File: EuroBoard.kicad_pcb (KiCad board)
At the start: 2 copper layers, 99.9 x 99.9 mm, 36 parts, among them J1 GPIO, J10 PD1, J11 PD2, J12 PD3, J2 Conn_01x07_Male, J3 I2C, J4 Conn_01x05_Male, J5 RX, J6 TX, J7 GND, SW1 RESET, SW2 SW_DIP_x04, U1 AMS1117-3.3, U2 STM32G030CxT, Y1 NX2520 16MHz

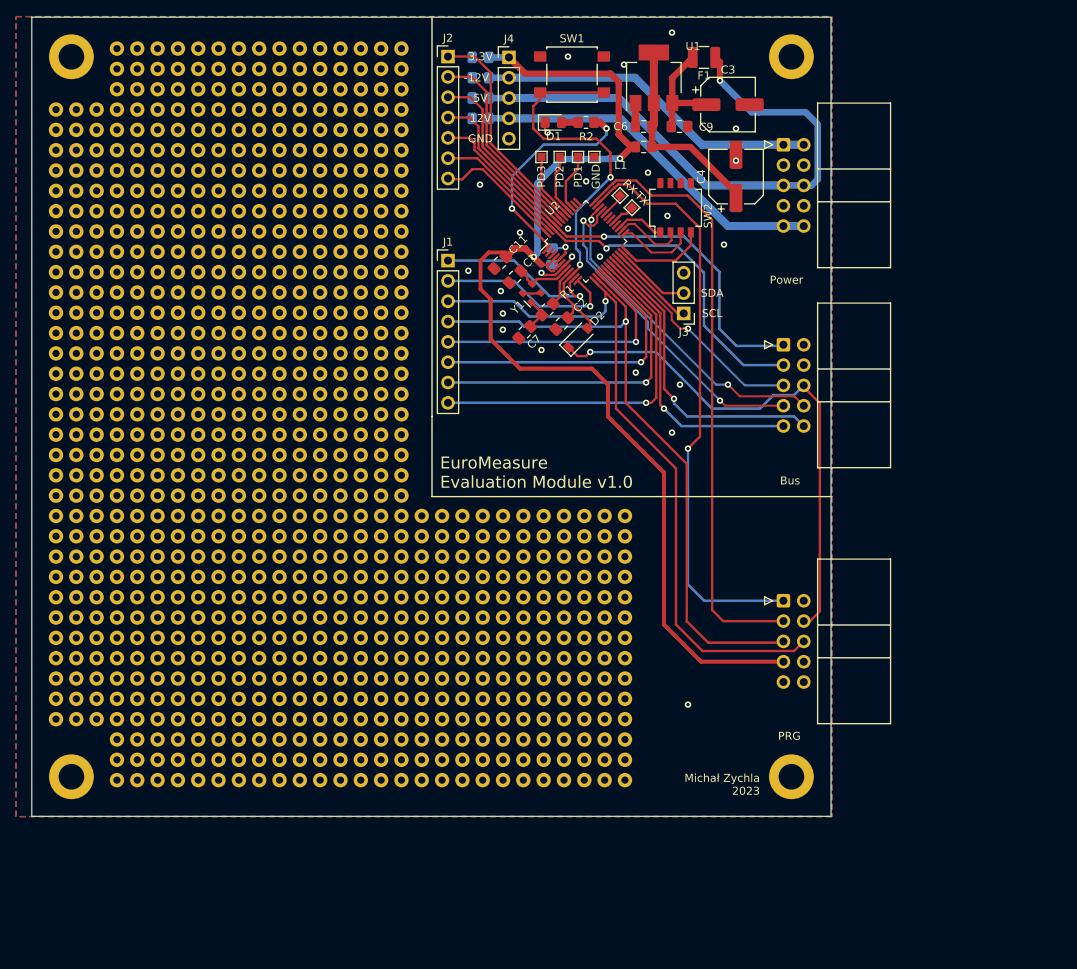
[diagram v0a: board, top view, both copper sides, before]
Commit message: Rework
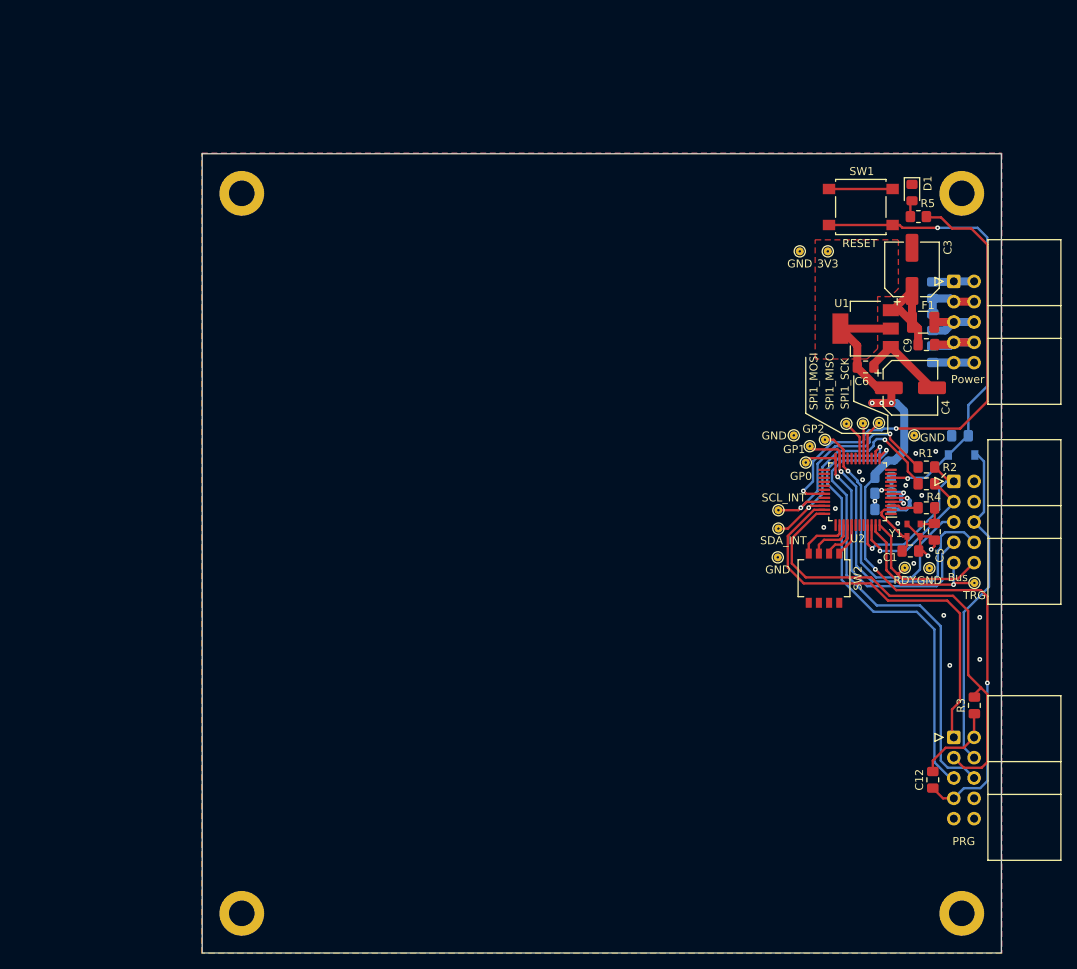
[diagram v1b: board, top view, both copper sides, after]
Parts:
- removed C11: 10u, Capacitor_SMD:C_0805_2012Metric_Pad1.18x1.45mm_HandSolder
- removed J1: GPIO, Connector_PinHeader_2.54mm:PinHeader_1x08_P2.54mm_Vertical
- removed J10: PD1, TestPoint:TestPoint_Pad_1.0x1.0mm
- removed J11: PD2, TestPoint:TestPoint_Pad_1.0x1.0mm
- removed J12: PD3, TestPoint:TestPoint_Pad_1.0x1.0mm
- removed J2: Conn_01x07_Male, Connector_PinHeader_2.54mm:PinHeader_1x07_P2.54mm_Vertical
- removed J3: I2C, Connector_PinHeader_2.54mm:PinHeader_1x03_P2.54mm_Vertical
- removed J4: Conn_01x05_Male, Connector_PinHeader_2.54mm:PinHeader_1x05_P2.54mm_Vertical
- removed J5: RX, TestPoint:TestPoint_Pad_1.0x1.0mm
- removed J6: TX, TestPoint:TestPoint_Pad_1.0x1.0mm
- removed J7: GND, TestPoint:TestPoint_Pad_1.0x1.0mm
- removed REF**: ProtoArea, MEMS_Custom:ProtoArea
- added C5: 8p, Capacitor_SMD:C_0805_2012Metric_Pad1.18x1.45mm_HandSolder, F.Cu at (187.8, 97.4)
- added R3: 10k, Capacitor_SMD:C_0805_2012Metric_Pad1.18x1.45mm_HandSolder, F.Cu at (192.8, 119.1)
- added R4: 0R, Capacitor_SMD:C_0805_2012Metric_Pad1.18x1.45mm_HandSolder, F.Cu at (186.8, 94.4)
- added R5: 1k, Resistor_SMD:R_0805_2012Metric_Pad1.20x1.40mm_HandSolder, F.Cu at (185.8, 58.0)
- added TP1: SPI1_SCK, MEMS_Custom:TestPoint_Pad_D1.0mm, F.Cu at (180.9, 83.8)
- added TP10: GP0, MEMS_Custom:TestPoint_Pad_D1.0mm, F.Cu at (171.7, 88.7)
- added TP11: GND, MEMS_Custom:TestPoint_Pad_D1.0mm, F.Cu at (168.2, 100.6)
- added TP12: GND, MEMS_Custom:TestPoint_Pad_D1.0mm, F.Cu at (187.2, 101.9)
- added TP13: GND, MEMS_Custom:TestPoint_Pad_D1.0mm, F.Cu at (171.0, 62.3)
- added TP14: GND, MEMS_Custom:TestPoint_Pad_D1.0mm, F.Cu at (170.2, 85.3)
- added TP15: GND, MEMS_Custom:TestPoint_Pad_D1.0mm, F.Cu at (185.3, 85.3)
- added TP16: 3V3, MEMS_Custom:TestPoint_Pad_D1.0mm, F.Cu at (174.5, 62.3)
- added TP2: SPI1_MISO, MEMS_Custom:TestPoint_Pad_D1.0mm, F.Cu at (178.9, 83.8)
- added TP3: SPI1_MOSI, MEMS_Custom:TestPoint_Pad_D1.0mm, F.Cu at (176.8, 83.9)
- added TP4: SCL_INT, MEMS_Custom:TestPoint_Pad_D1.0mm, F.Cu at (168.3, 94.7)
- added TP5: SDA_INT, MEMS_Custom:TestPoint_Pad_D1.0mm, F.Cu at (168.3, 97.0)
- added TP6: TRG, MEMS_Custom:TestPoint_Pad_D1.0mm, F.Cu at (192.8, 103.8)
- added TP7: RDY, MEMS_Custom:TestPoint_Pad_D1.0mm, F.Cu at (184.1, 101.9)
- added TP8: GP2, MEMS_Custom:TestPoint_Pad_D1.0mm, F.Cu at (174.1, 85.9)
- added TP9: GP1, MEMS_Custom:TestPoint_Pad_D1.0mm, F.Cu at (172.2, 86.7)
- C1: value C -> 8p
- C12: moved to F.Cu
- C2, D2, L1: moved to B.Cu
- C7: value C -> 100n; moved to B.Cu
- C8: value 100n -> 10u
- R1: value R -> 0R; footprint Resistor_SMD:R_0805_2012Metric_Pad1.20x1.40mm_HandSolder -> Capacitor_SMD:C_0805_2012Metric_Pad1.18x1.45mm_HandSolder
- R2: value 1k -> 0R; footprint Resistor_SMD:R_0805_2012Metric_Pad1.20x1.40mm_HandSolder -> Capacitor_SMD:C_0805_2012Metric_Pad1.18x1.45mm_HandSolder
- moved C12 106.5 mm to (187.6, 128.4), turned to 90 degrees
- moved C15 63.8 mm to (187.6, 75.2), turned to 90 degrees
- moved C14 63.1 mm to (187.6, 71.2), turned to 90 degrees
- moved C13 62.5 mm to (187.6, 67.2), turned to -90 degrees
- moved R2 62.1 mm to (186.8, 91.4)
- moved C1 60.1 mm to (184.8, 99.8), turned to 0 degrees
- moved Y1 56.2 mm to (185.2, 97.2), turned to 180 degrees
- moved C2 51.7 mm to (191.0, 85.4), turned to 180 degrees
- moved R1 51.3 mm to (186.8, 89.3), turned to 180 degrees
- moved L1 51.0 mm to (181.4, 90.6), turned to 0 degrees
- moved C8 50.9 mm to (181.4, 92.6), turned to 180 degrees
- moved D2 50.1 mm to (191.2, 87.8), turned to 180 degrees
- moved C7 50.0 mm to (181.4, 94.6), turned to 180 degrees
- moved SW2 49.9 mm to (174.0, 103.2), turned to -90 degrees
- moved U2 46.2 mm to (178.2, 92.4), turned to 180 degrees
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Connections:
- B1 pad 11: /SCL -> /SCL_EXT
- B1 pad 13: /SDA -> /SDA_EXT
- C1 pad 1: /OSC_IN -> Net-(U2-Pad2)
- C4 pad 1: Net-(C4-Pad1) -> +3.3V
- C6 pad 1: Net-(C4-Pad1) -> +3.3V
- C7 pad 1: Net-(C7-Pad1) -> Net-(U2-Pad5)
- C8 pad 1: /VREF -> Net-(L1-Pad2)
- L1 pad 1: Net-(C4-Pad1) -> +3.3V
- L1 pad 2: +3.3V -> Net-(L1-Pad2)
- R1 pad 1: Net-(C7-Pad1) -> /SCL_EXT
- R1 pad 2: /OSC_OUT -> /SCL_INT
- R2 pad 1: Net-(D1-Pad2) -> /SDA_INT
- R2 pad 2: /LED -> /SDA_EXT
- SW2 pad 1: Net-(SW2-Pad1) -> Net-(U2-Pad41)
- SW2 pad 2: Net-(SW2-Pad2) -> Net-(U2-Pad40)
- SW2 pad 3: Net-(SW2-Pad3) -> Net-(U2-Pad39)
- SW2 pad 4: Net-(SW2-Pad4) -> Net-(U2-Pad38)
- U1 pad 2: Net-(C4-Pad1) -> +3.3V
- U2 pad 1: /LED -> /PC13
- U2 pad 11: Net-(J1-Pad1) -> /PA0
- U2 pad 12: /SPI1_SCK -> /PA1
- U2 pad 15: Net-(J1-Pad5) -> /PA4
- U2 pad 16: Net-(J1-Pad6) -> /SPI1_SCK
- U2 pad 19: /TRG -> /PB0
- U2 pad 2: unconnected-(U2-Pad2) -> Net-(U2-Pad2)
- U2 pad 20: /RDY -> /PB1
- U2 pad 21: /GP2 -> /PB2
- U2 pad 22: /SCL2 -> /GP2
- U2 pad 23: /SDA2 -> /GP1
- U2 pad 24: Net-(SW2-Pad4) -> /GP0
- U2 pad 25: Net-(SW2-Pad3) -> /SPI2_SCK
- U2 pad 26: Net-(SW2-Pad2) -> /SPI2_MISO
- U2 pad 27: Net-(SW2-Pad1) -> /SPI2_MOSI
- U2 pad 28: unconnected-(U2-Pad28) -> /PA8
- U2 pad 29: /TX_AUX -> /PA9
- U2 pad 3: unconnected-(U2-Pad3) -> Net-(U2-Pad3)
- U2 pad 30: unconnected-(U2-Pad30) -> /PB6
- U2 pad 31: unconnected-(U2-Pad31) -> Net-(U2-Pad31)
- U2 pad 32: /RX_AUX -> /PA10
- U2 pad 33: /GP0 -> /SCL_INT
- U2 pad 34: /GP1 -> /SDA_INT
- U2 pad 37: unconnected-(U2-Pad37) -> /PA15
- U2 pad 38: unconnected-(U2-Pad38) -> Net-(U2-Pad38)
- U2 pad 4: +3.3V -> Net-(L1-Pad2)
- U2 pad 40: Net-(J11-Pad1) -> Net-(U2-Pad40)
- U2 pad 41: Net-(J12-Pad1) -> Net-(U2-Pad41)
- U2 pad 42: Net-(J2-Pad1) -> /PB3
- U2 pad 43: Net-(J2-Pad2) -> /PB4
- U2 pad 44: Net-(J2-Pad3) -> /PB5
- U2 pad 45: /SCL -> /SCL_EXT
- U2 pad 46: /SDA -> /SDA_EXT
- U2 pad 47: Net-(J2-Pad6) -> /TRG
- U2 pad 48: Net-(J2-Pad7) -> /RDY
- U2 pad 5: /VREF -> Net-(U2-Pad5)
- U2 pad 6: +3.3V -> Net-(L1-Pad2)
- U2 pad 8: /OSC_IN -> /PF0
- U2 pad 9: /OSC_OUT -> /PF1
- Y1 pad 1: Net-(C7-Pad1) -> Net-(Y1-Pad1)
- Y1 pad 3: /OSC_IN -> Net-(U2-Pad2)
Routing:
- net +5V: track 70.5 -> 8.04 mm, vias 1 -> 0
- net Net-(U2-Pad31): track 0.00 -> 60.9 mm, vias 0 -> 2
- net /SCL: track 59.6 -> 0.00 mm, vias 1 -> 0
- net /SDA: track 58.4 -> 0.00 mm, vias 1 -> 0
- net GND: track 12.1 -> 59.0 mm, vias 25 -> 19
- net +3.3V: track 141.7 -> 95.4 mm, vias 2 -> 5
- net /SPI1_MOSI: track 45.2 -> 5.02 mm, vias 1 -> 0
- net +12V: track 44.9 -> 5.17 mm
- net Net-(J1-Pad6): track 37.9 -> 0.00 mm, vias 1 -> 0
- net -12V: track 42.8 -> 5.19 mm
- net /SPI1_MISO: track 41.6 -> 4.42 mm, vias 1 -> 0
- net Net-(J1-Pad5): track 33.8 -> 0.00 mm, vias 1 -> 0
- net /SDA_INT: track 0.00 -> 29.5 mm, vias 0 -> 2
- net /SCL_INT: track 0.00 -> 29.0 mm, vias 0 -> 2
- net /TX_DEBUG: track 88.2 -> 59.5 mm
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- added copper zone on F.Cu, net +3.3V
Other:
- board text removed: "-12V"
- board text removed: "12V"
- board text removed: "3.3V"
- board text removed: "5V"
- board text removed: "EuroMeasure Evaluation Module v1.0"
- board text removed: "GND"
- board text removed: "Michał Zychla 2023"
- board text removed: "SCL"
- board text removed: "SDA"
